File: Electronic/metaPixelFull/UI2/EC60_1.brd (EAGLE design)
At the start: 66 x 65.7 mm, 4 parts

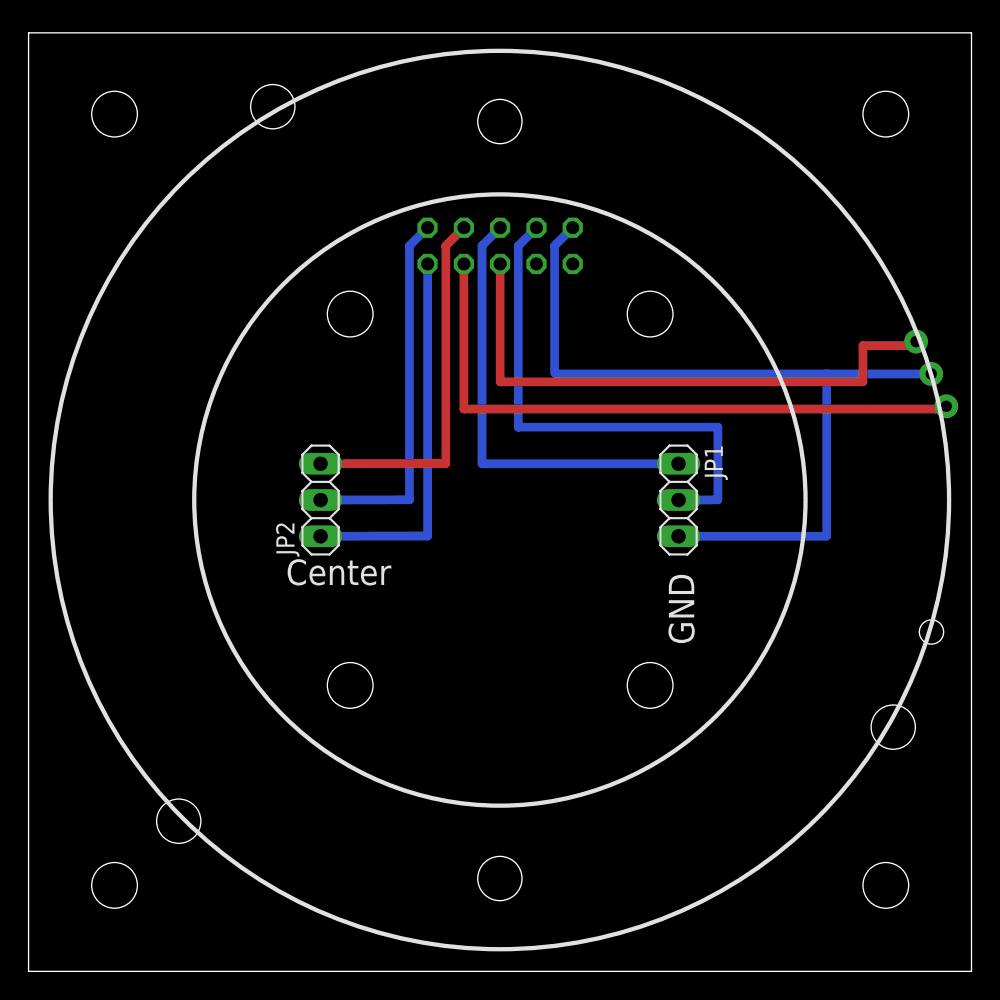
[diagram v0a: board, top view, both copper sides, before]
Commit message: Building the UI-Board
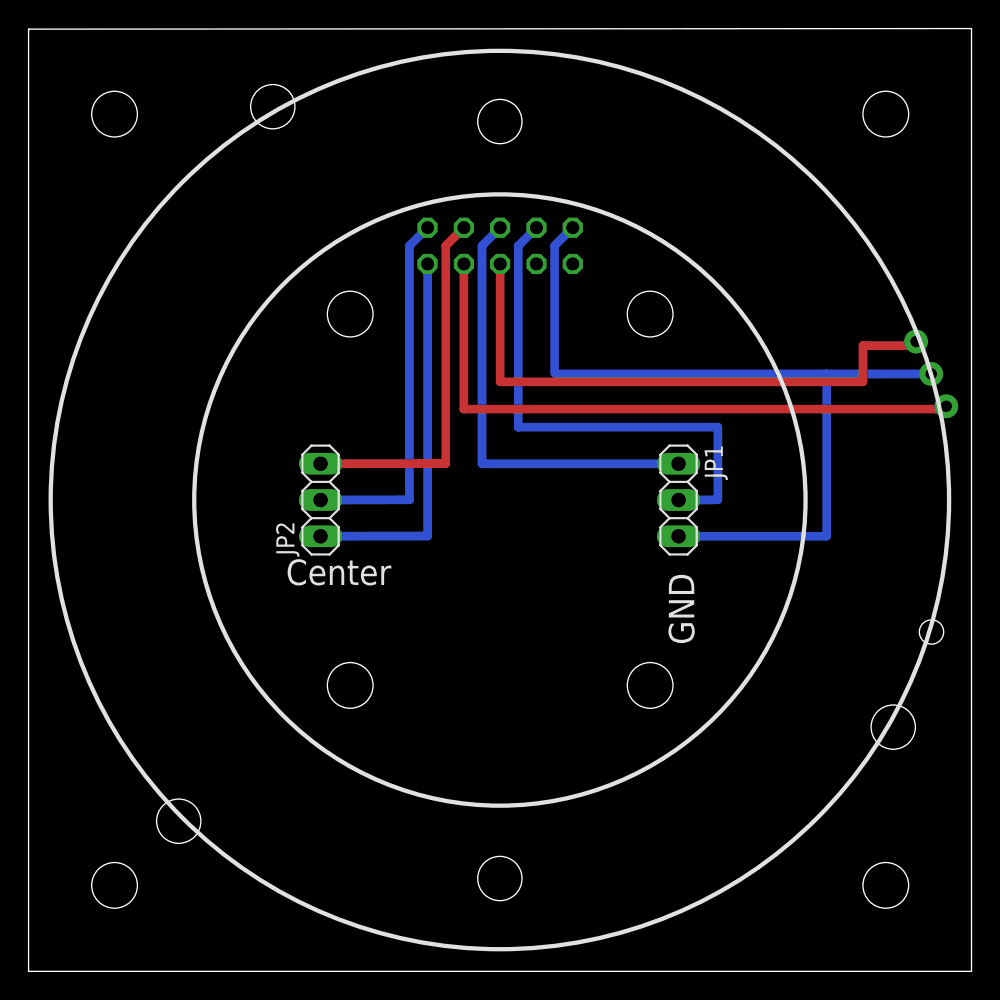
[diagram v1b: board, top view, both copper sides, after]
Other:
- board size 66 x 65.7 mm -> 66 x 66 mm
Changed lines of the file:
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@@
 <setting verticaltext="up"/>
 </settings>
-<grid distance="0.1" unitdist="inch" unit="mil" style="lines" multiple="1" display="yes" altdistance="0.05" altunitdist="inch" altunit="mil"/>
+<grid distance="1" unitdist="mm" unit="mm" style="lines" multiple="1" display="yes" altdistance="0.1" altunitdist="mm" altunit="mm"/>
 <layers>
 <layer number="1" name="Top" color="4" fill="1" visible="yes" active="yes"/>
@@
 <plain>
 <wire x1="0" y1="0" x2="66.02" y2="0" width="0" layer="20"/>
-<wire x1="66.02" y1="0" x2="66.02" y2="65.71" width="0" layer="20"/>
-<wire x1="66.02" y1="65.71" x2="0" y2="65.71" width="0" layer="20"/>
-<wire x1="0" y1="65.71" x2="0" y2="0" width="0" layer="20"/>
+<wire x1="66.02" y1="0" x2="66.02" y2="66.01" width="0" layer="20"/>
+<wire x1="66.02" y1="66.01" x2="0" y2="65.97" width="0" layer="20"/>
+<wire x1="0" y1="65.97" x2="0" y2="0" width="0" layer="20"/>
 <hole x="22.52" y="46.02" drill="3.2"/>
 <hole x="43.52" y="46.02" drill="3.2"/>
